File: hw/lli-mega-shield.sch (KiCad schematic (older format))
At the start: 23 parts

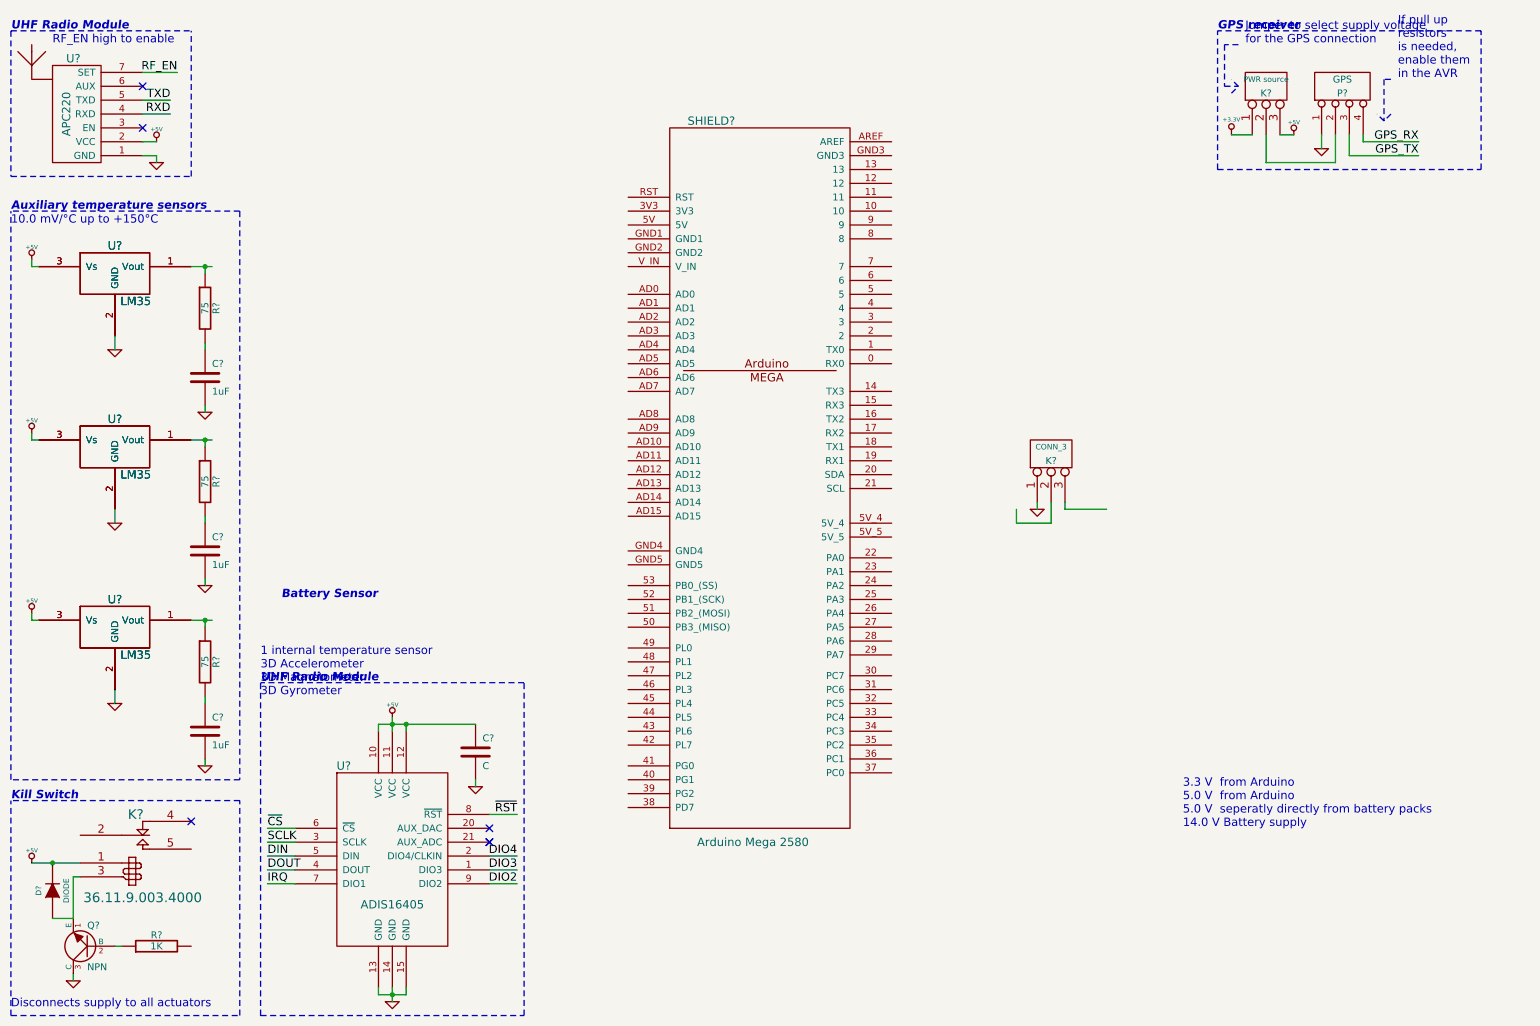
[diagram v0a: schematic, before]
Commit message: Added more electronics
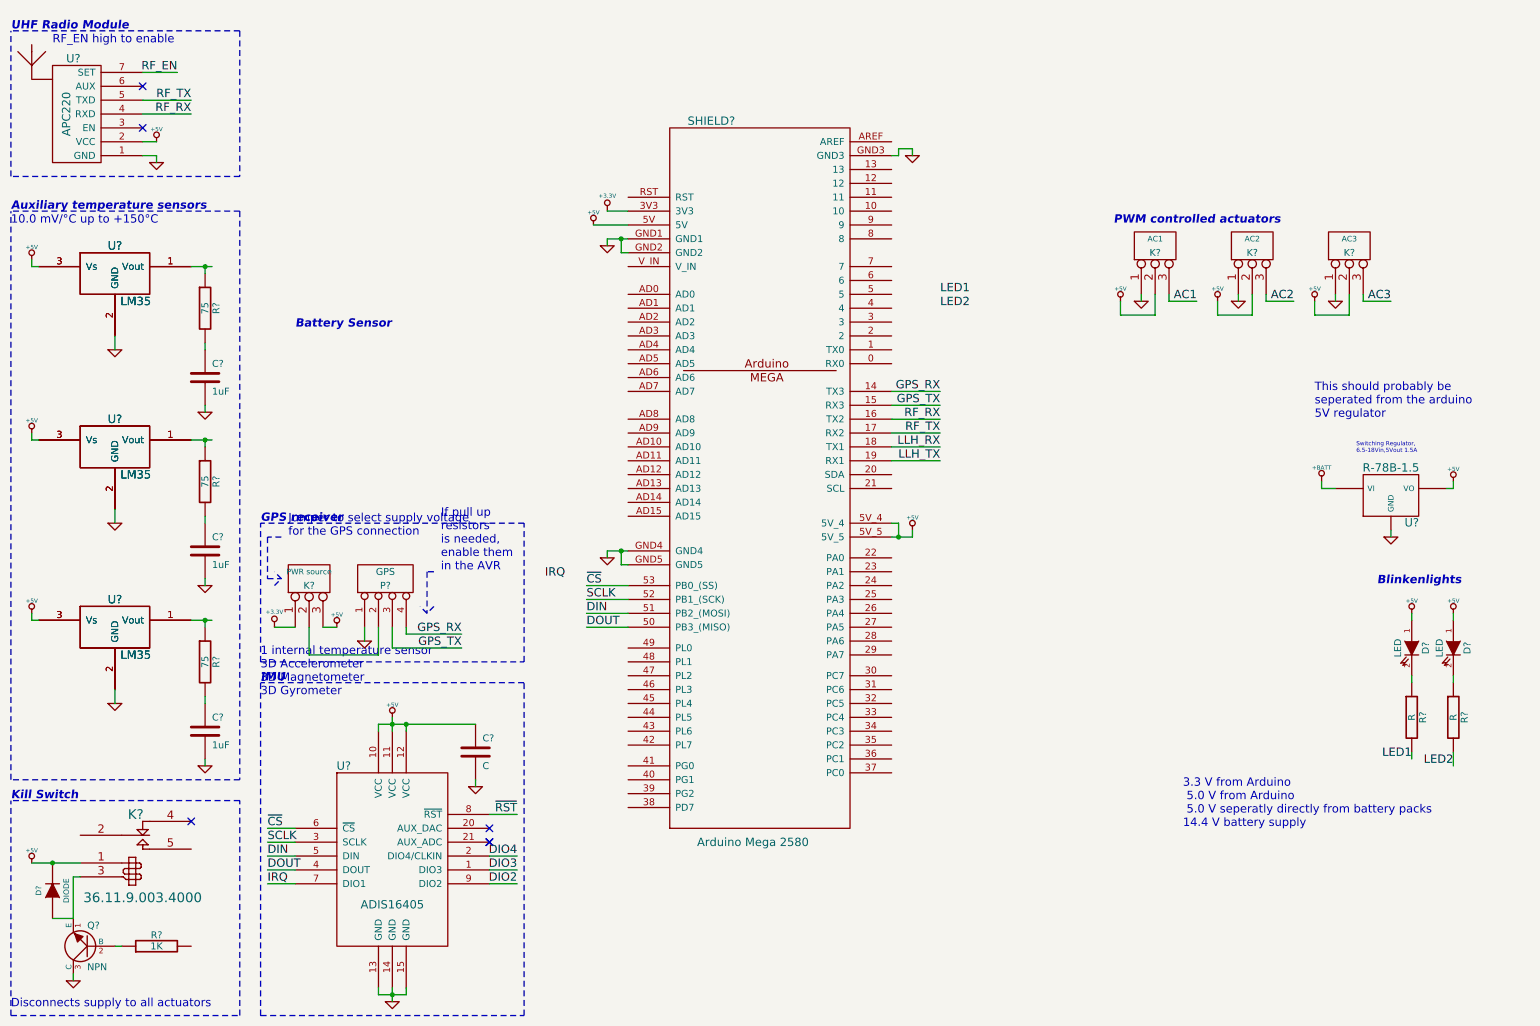
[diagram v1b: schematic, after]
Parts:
- added D? (x2): LED, symbol LED
- added K?: AC1, symbol CONN_3
- added K?: AC3, symbol CONN_3
- added R? (x2): R, symbol R
- added U?: R-78B-1.5, symbol 7805
- K?: value CONN_3 -> AC2
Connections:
- net labels added: +BATT, AC1, AC2, AC3, LED1, LED2, LLH_RX, LLH_TX, RF_RX, RF_TX
- net labels removed: RXD, TXD
- wire segments 67 -> 118
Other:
- note added: "3.3 V from Arduino\n 5.0 V from Arduino\n 5.0 V seperatly directly from battery packs\n14.4 V battery supply"
- note added: "Blinkenlights"
- note added: "IMU"
- note added: "PWM controlled actuators"
- note added: "Switching Regulator,\n6.5-18Vin,5Vout 1.5A"
- note added: "This should probably be\nseperated from the arduino\n5V regulator"
- note removed: "3.3 V from Arduino\n5.0 V from Arduino\n5.0 V seperatly directly from battery packs\n14.0 V Battery supply"
- moved on the sheet: K?, P?

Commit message: More hardware before I go home
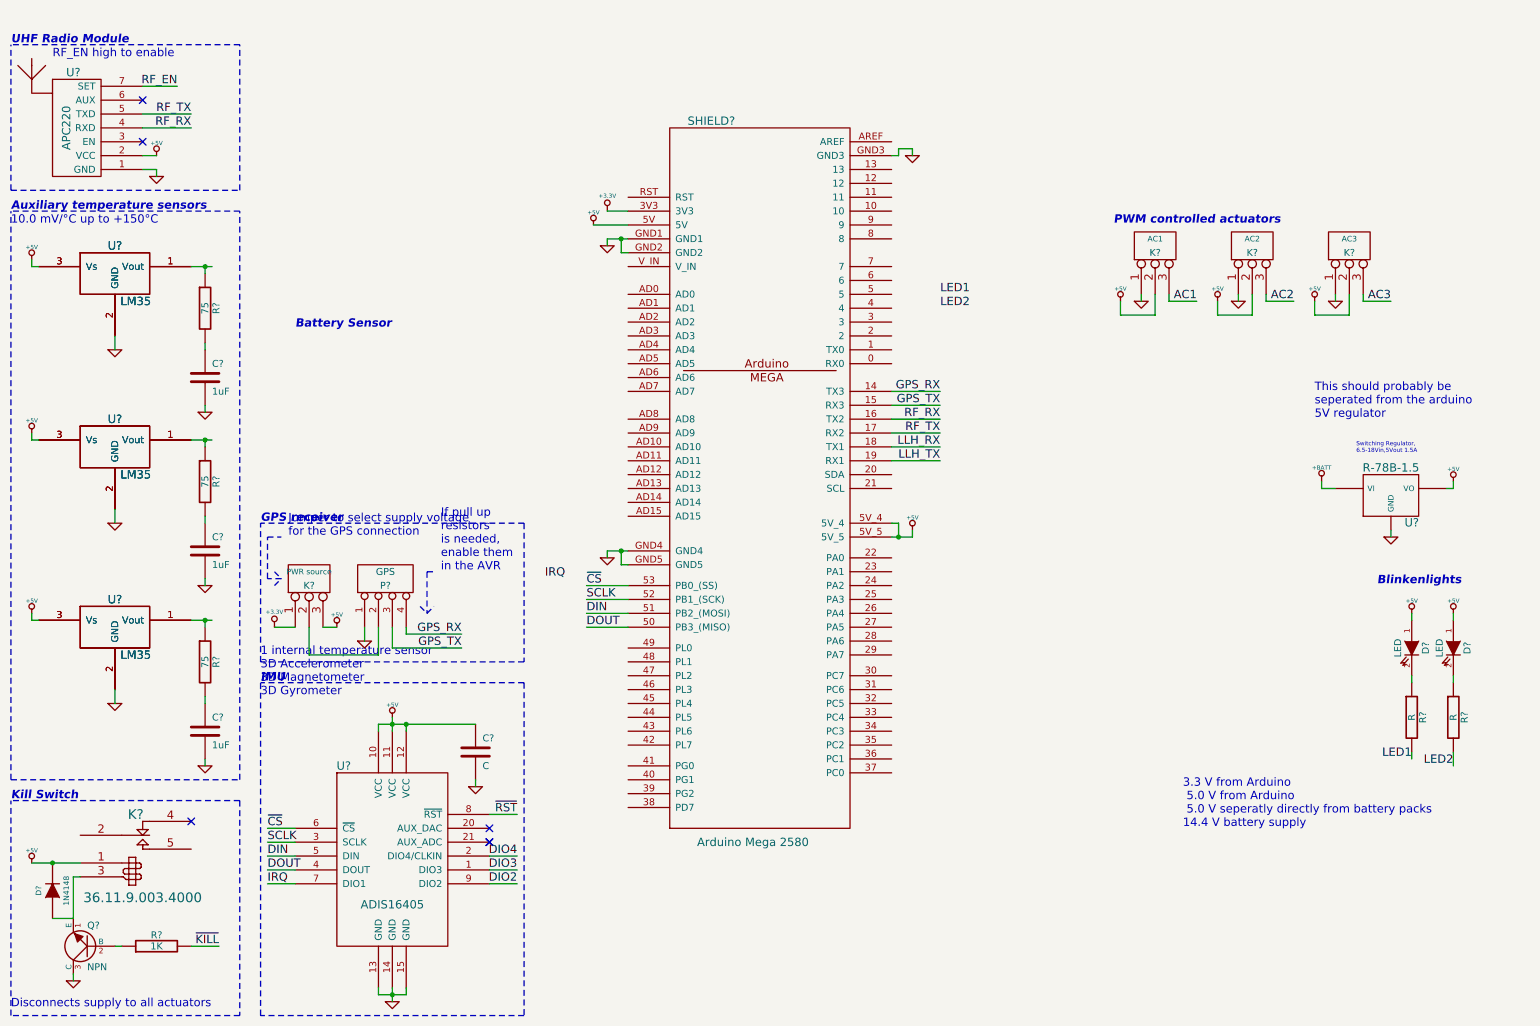
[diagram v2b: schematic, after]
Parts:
- D?: value DIODE -> 1N4148
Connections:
- net ~KILL: now reaches R?.2
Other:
- moved on the sheet: U?
